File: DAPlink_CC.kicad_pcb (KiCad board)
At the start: 6 copper layers, 34 x 12.5 mm, 89 parts, among them J1 USB_TypeC-24, J2 Conn_01x04, J3 USB_TypeC-24, J4 Conn_01x02, J5 Conn_01x02, J6 Conn_01x04, Q1 YJL2101W, Q2 TPM7002DFN3, U1 ZD25Q80BNIGR, U10 DIO32220LP10, U11 AW33901FCR, U2 SL2.1S, U3 GD32F350G8U6, U4 LP5240HVF, U5 JW5393FSOTI, U6 HC32L110B6YA, U7 LP5240HVF, U8 DIO32220LP10, U9 DIO32220LP10, X1 12MHz

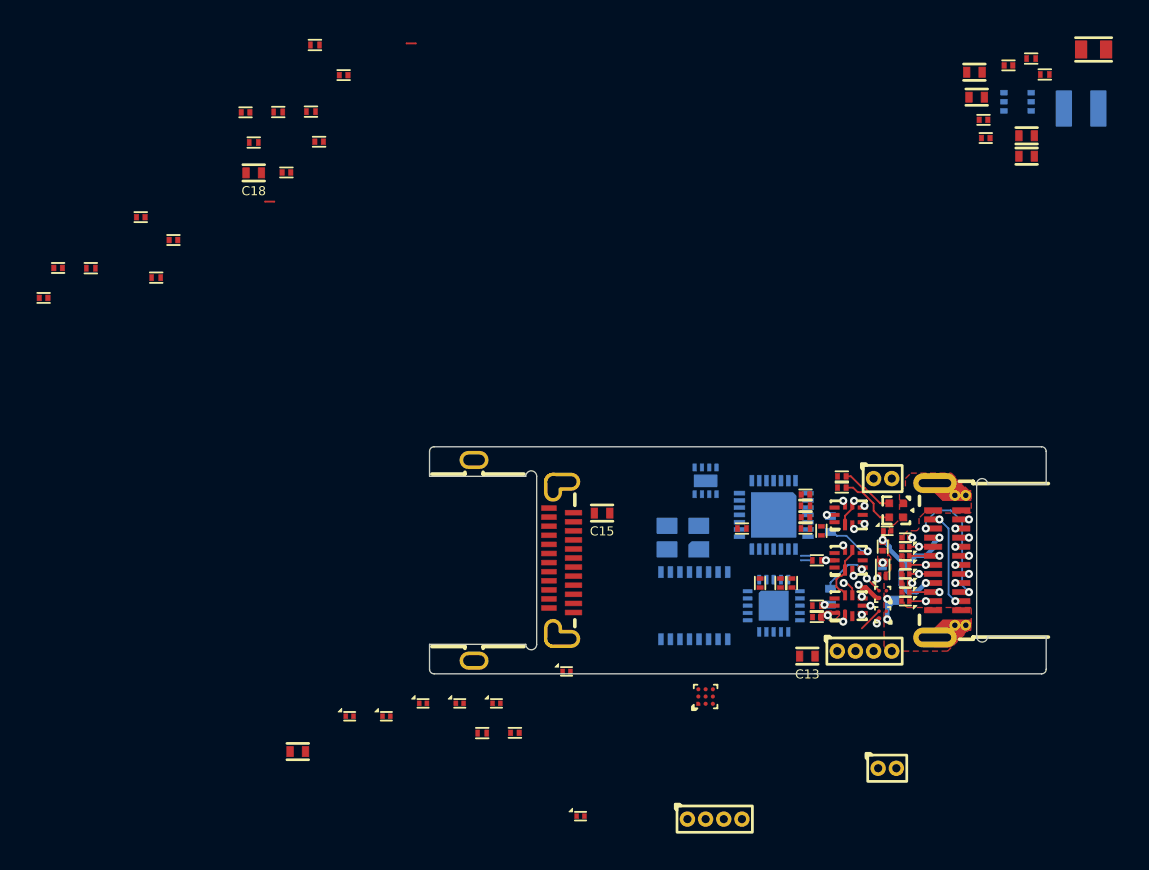
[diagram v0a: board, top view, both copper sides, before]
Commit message: Daily update
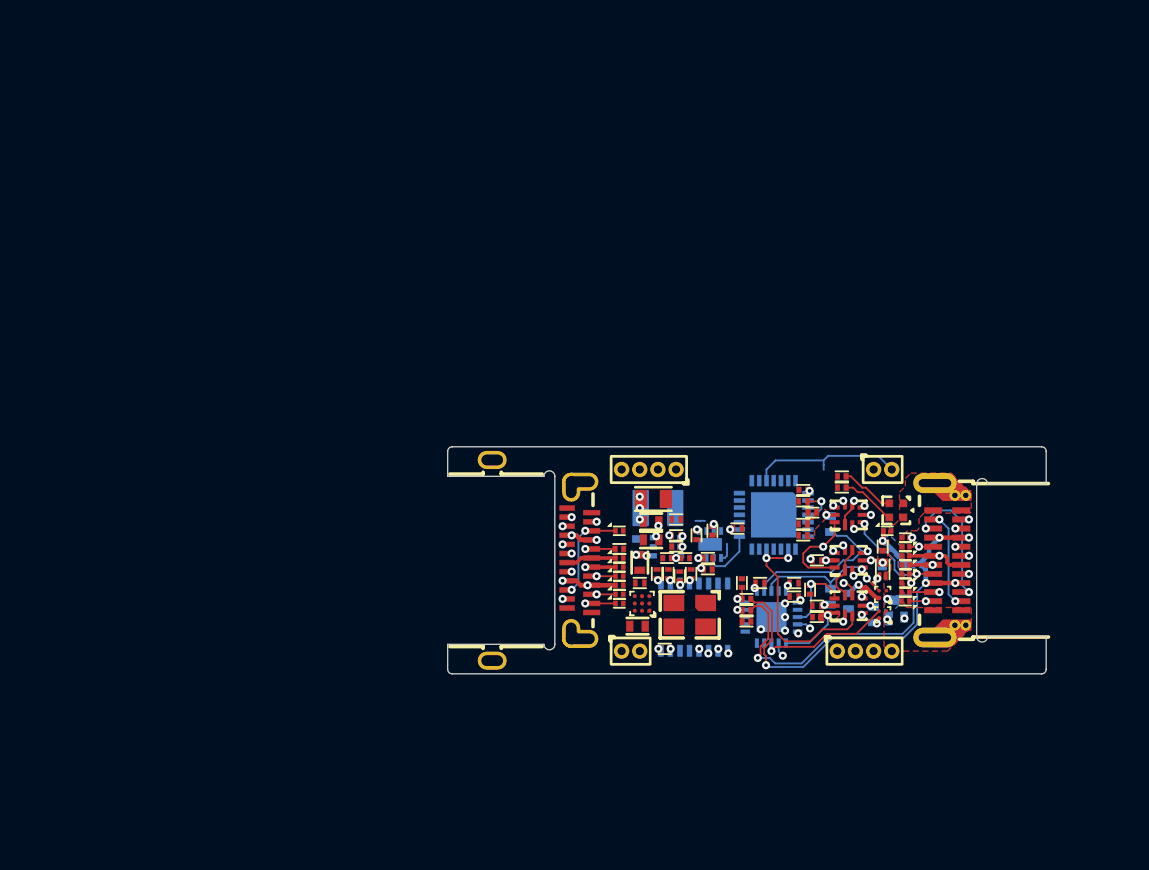
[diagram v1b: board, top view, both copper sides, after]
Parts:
- C13, C15, C18, C9, NT1, NT2: moved to B.Cu
- NT4, X1: moved to F.Cu
- moved C18 43.0 mm to (116.8, 103.1)
- moved R15 40.0 mm to (112.0, 101.6), turned to 90 degrees
- moved R6 39.8 mm to (108.5, 102.8), turned to 180 degrees
- moved R4 39.4 mm to (106.4, 100.5)
- moved R7 39.3 mm to (108.5, 103.4)
- moved R3 39.0 mm to (106.6, 98.4), turned to -90 degrees
- moved C1 37.1 mm to (105.5, 100.8), turned to -90 degrees
- moved C5 35.9 mm to (104.0, 104.9), turned to 180 degrees
- moved R9 35.5 mm to (108.2, 101.2), turned to 90 degrees
- moved C3 34.7 mm to (103.6, 100.8), turned to 90 degrees
- moved FB1 34.6 mm to (103.4, 96.6), turned to 180 degrees
- moved R8 34.5 mm to (108.5, 102.1), turned to 180 degrees
- moved C2 34.1 mm to (106.4, 99.9)
- moved C4 33.3 mm to (104.2, 100.8), turned to 90 degrees
- moved C10 32.7 mm to (102.6, 100.1), turned to -90 degrees
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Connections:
- U6 pad 16: (no net) -> unconnected-(U6-Pad16)
- U6 pad 17: (no net) -> unconnected-(U6-Pad17)
- U6 pad 18: (no net) -> unconnected-(U6-Pad18)
- U6 pad 7: (no net) -> unconnected-(U6-Pad7)
- U6 pad EP: (no net) -> GND
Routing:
- net /SWDIO_TMS: track 6.92 -> 24.8 mm
- net /DVC-DP: track 2.39 -> 20.2 mm
- net VDC: track 11.3 -> 28.8 mm, vias 5 -> 6
- net /DVC-DN: track 4.60 -> 19.7 mm, vias 2 -> 3
- net VDD: track 1.71 -> 16.2 mm, vias 2 -> 3
- net /3V3_SEL: track 0.95 -> 12.8 mm, vias 1 -> 2
- net /SWCLK_TCK: track 6.13 -> 17.1 mm
- net /DIR_SEL: track 0.00 -> 10.8 mm, vias 0 -> 2
- net /SWO_TDO: track 0.00 -> 10.4 mm, vias 0 -> 1
- net /~{OE}: track 0.00 -> 9.28 mm, vias 0 -> 3
- net /DAP_Tx: track 0.00 -> 9.20 mm, vias 0 -> 3
- net /DAP_CLK: track 0.00 -> 8.83 mm, vias 0 -> 3
- net /TRST: track 0.00 -> 8.13 mm
- net /DAP_Rx: track 0.00 -> 7.52 mm, vias 0 -> 4
- net /IDL-D: track 0.00 -> 6.96 mm, vias 1 -> 2
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- added copper zone on F.Cu, net +3V3
- added copper zone on B.Cu, net VDC
- added copper zone on B.Cu, net VDD
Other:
- board size 34 x 12.5 mm -> 33 x 12.5 mm
